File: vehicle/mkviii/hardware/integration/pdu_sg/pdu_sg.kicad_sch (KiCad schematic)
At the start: 2 parts, among them U2 MCP23S17-E_SO, U3 STM32G441KBT6

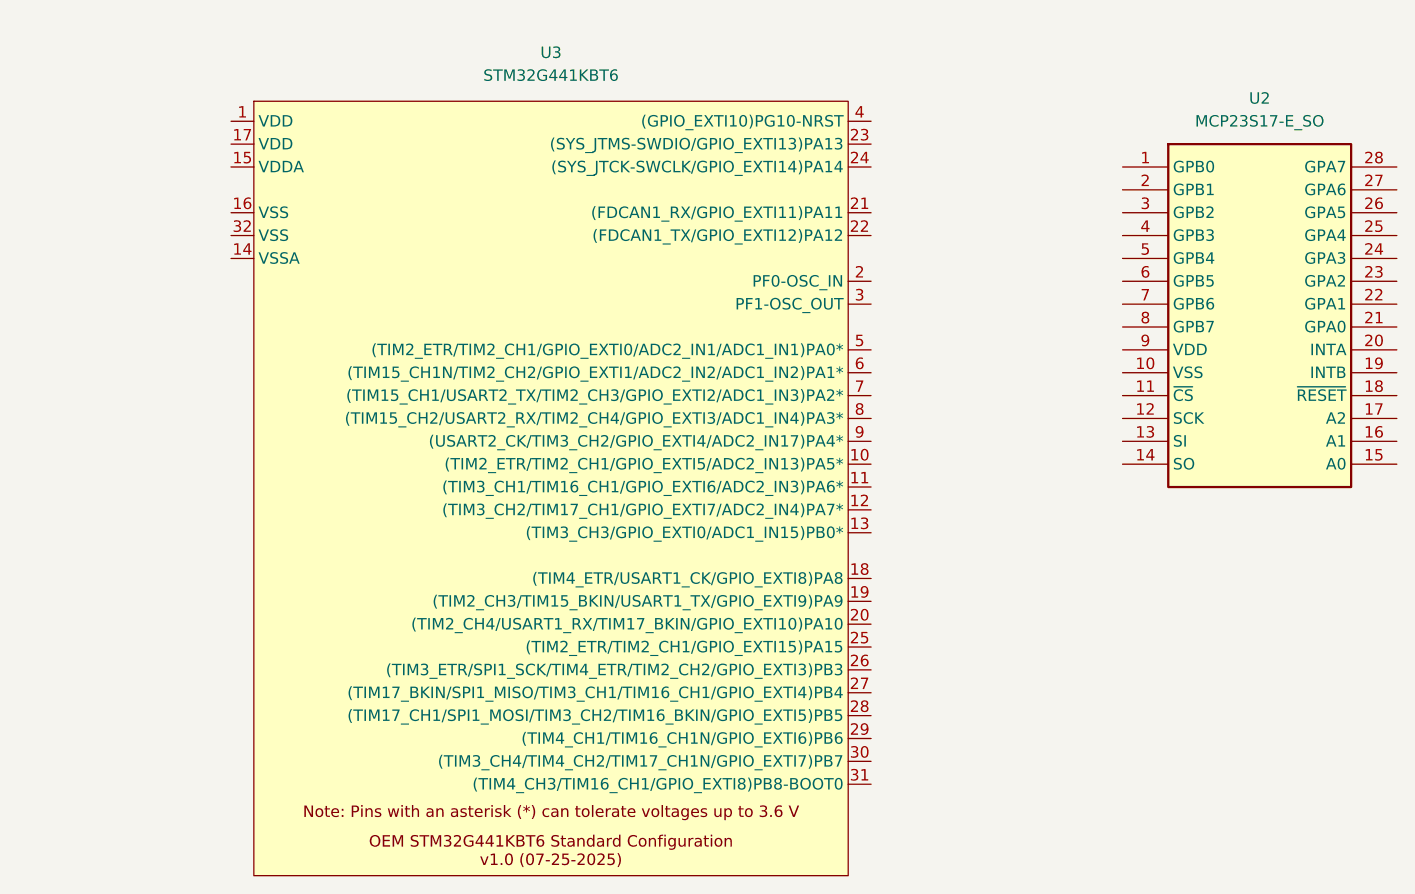
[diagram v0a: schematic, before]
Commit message: power
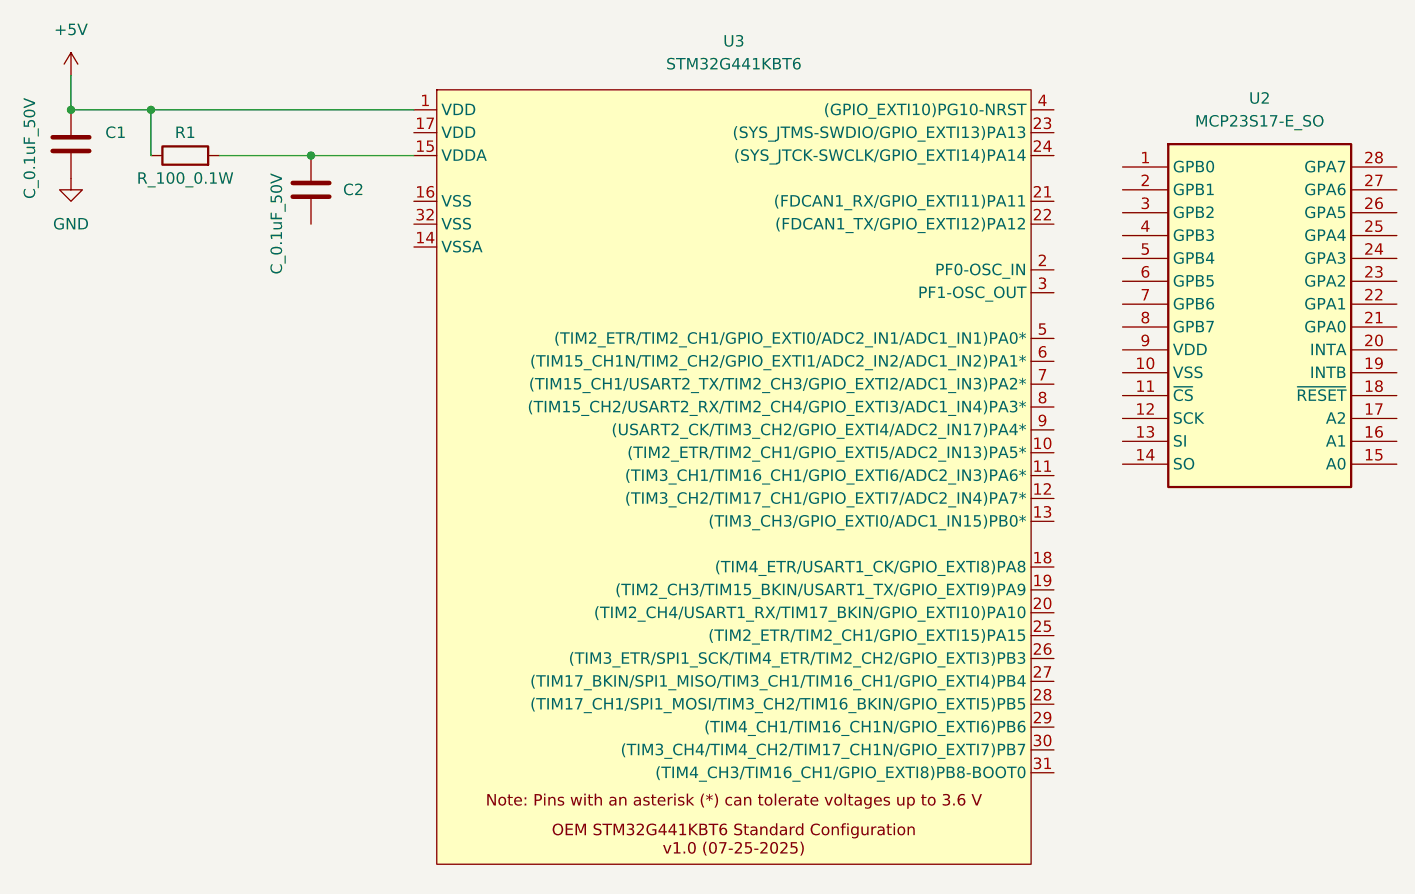
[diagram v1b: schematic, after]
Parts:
- added C1, C2: C_0.1uF_50V, OEM:C_0603_1608Metric, symbol OEM:C_0.1uF_50V_0603
- added R1: R_100_0.1W, OEM:R_0603_1608Metric, symbol OEM:R_100_0.1W_0603
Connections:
- net +5V: now reaches U3.1 (VDD)
- net +5V: now also C1.1, R1.1
- net at U3.15 (VDDA): now also C2.1, R1.2
- new net GND: C1.2
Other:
- moved on the sheet: U3
